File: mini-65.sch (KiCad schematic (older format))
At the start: 170 parts, among them J1 TYPE-C-31-M12_13_EDITED, J2 AVR-ISP-6, SW1 SW_Push, U1 ATmega32U4-AU, U2 USBLC6-2SC6, Y1 Crystal_GND24_Small

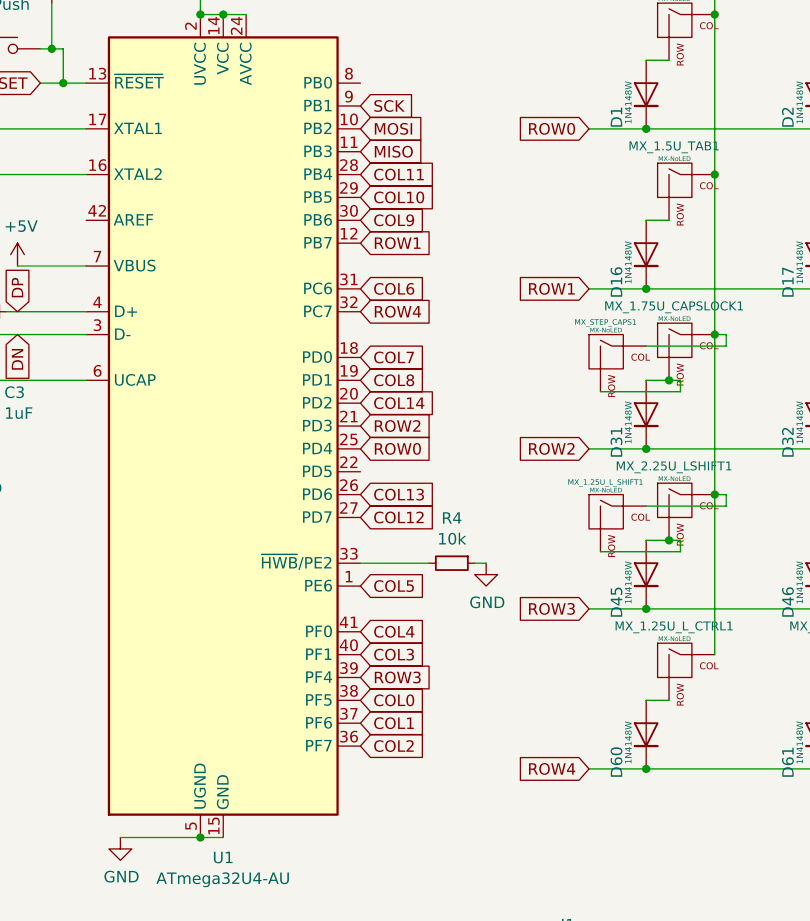
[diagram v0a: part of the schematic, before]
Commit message: misc changes, including ICSP silkscreen
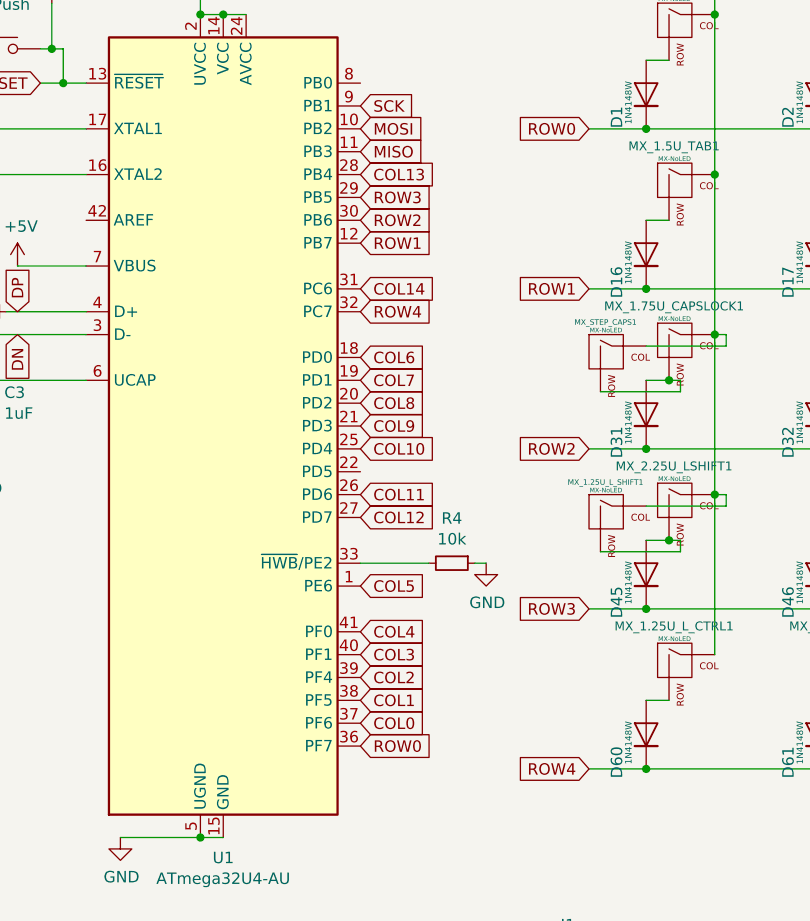
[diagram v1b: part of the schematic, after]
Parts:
- J2: footprint mini-general-tweaks:PinHeader_2x03_P2.54mm_Vertical_ICSP -> mini-general-tweaks:ICSP_2.54mm_LAYOUT
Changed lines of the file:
@@
 F 0 "J2" H 921 6596 50  0000 R CNN
 F 1 "AVR-ISP-6" H 921 6505 50  0000 R CNN
-F 2 "mini-general-tweaks:PinHeader_2x03_P2.54mm_Vertical_ICSP" V 950 6550 50  0001 C CNN
+F 2 "mini-general-tweaks:ICSP_2.54mm_LAYOUT" V 950 6550 50  0001 C CNN
 F 3 " ~" H -75 5950 50  0001 C CNN
 	1    1200 6500
@@
 	1    0    0    -1
 $EndComp
-Connection ~ 2450 1050
 Wire Wire Line
 	4200 2700 4550 2700
@@
 Wire Wire Line
 	8550 6350 8550 6400
-Text GLabel 3150 2950 2    50   Input ~ 0
-ROW0
-Text GLabel 3150 2050 2    50   Input ~ 0
-ROW1
-Text GLabel 3150 2850 2    50   Input ~ 0
-ROW2
-Text GLabel 3150 2750 2    50   Input ~ 0
-COL14
-Text GLabel 3150 3150 2    50   Input ~ 0
-COL13
-Text GLabel 3150 3250 2    50   Input ~ 0
-COL12
-Text GLabel 3150 1750 2    50   Input ~ 0
-COL11
-Text GLabel 3150 1850 2    50   Input ~ 0
-COL10
-Text GLabel 3150 1950 2    50   Input ~ 0
-COL9
-Text GLabel 3150 2650 2    50   Input ~ 0
-COL8
-Text GLabel 3150 2550 2    50   Input ~ 0
-COL7
-Text GLabel 3150 2250 2    50   Input ~ 0
-COL6
-Text GLabel 3150 2350 2    50   Input ~ 0
-ROW4
 Connection ~ 5450 3150
 Connection ~ 6500 3650
-Connection ~ 2550 1050
-Wire Wire Line
-	2650 1050 2550 1050
-Wire Wire Line
-	2550 1050 2450 1050
 Connection ~ 8300 4350
-Text GLabel 3150 4250 2    50   Input ~ 0
-COL2
-Text GLabel 3150 4150 2    50   Input ~ 0
-COL1
-Text GLabel 3150 4050 2    50   Input ~ 0
-COL0
-Text GLabel 3150 3950 2    50   Input ~ 0
-ROW3
-Text GLabel 3150 3850 2    50   Input ~ 0
-COL3
-Text GLabel 3150 3750 2    50   Input ~ 0
-COL4
-Text GLabel 3150 3550 2    50   Input ~ 0
-COL5
 Wire Wire Line
 	5450 3150 5450 3850
@@
 	5900 3650 6500 3650
 Connection ~ 4400 3650
-$Comp
-L MCU_Microchip_ATmega:ATmega32U4-AU U1
-U 1 1 5F16167A
-P 2550 2850
-F 0 "U1" H 2550 961 50  0000 C CNN
-F 1 "ATmega32U4-AU" H 2550 870 50  0000 C CNN
-F 2 "mini-general-tweaks:TQFP-44_10x10mm_P0.8mm_ATmega32U4" H 2550 2850 50  0001 C CIN
-F 3 "http://ww1.microchip.com/downloads/en/DeviceDoc/Atmel-7766-8-bit-AVR-ATmega16U4-32U4_Datasheet.pdf" H 2550 2850 50  0001 C CNN
-	1    2550 2850
-	1    0    0    -1
-$EndComp
 Wire Wire Line
 	3150 3450 3450 3450
-Connection ~ 2450 4650
-Wire Wire Line
-	2550 4650 2450 4650
-Wire Wire Line
-	2450 4650 2100 4650
 Connection ~ 5150 3650
 Wire Wire Line
@@
 	1    0    0    -1
 $EndComp
+Text GLabel 3150 3550 2    50   Input ~ 0
+COL5
+Text GLabel 3150 3750 2    50   Input ~ 0
+COL4
+Text GLabel 3150 3850 2    50   Input ~ 0
+COL3
+Text GLabel 3150 1850 2    50   Input ~ 0
+ROW3
+Text GLabel 3150 4050 2    50   Input ~ 0
+COL1
+Text GLabel 3150 4150 2    50   Input ~ 0
+COL0
+Text GLabel 3150 3950 2    50   Input ~ 0
+COL2
+Wire Wire Line
+	2450 4650 2100 4650
+Wire Wire Line
+	2550 4650 2450 4650
+Connection ~ 2450 4650
+Wire Wire Line
+	2550 1050 2450 1050
+Wire Wire Line
+	2650 1050 2550 1050
+Connection ~ 2550 1050
+Connection ~ 2450 1050
+Text GLabel 3150 4250 2    50   Input ~ 0
+ROW0
+Text GLabel 3150 2050 2    50   Input ~ 0
+ROW1
+Text GLabel 3150 1950 2    50   Input ~ 0
+ROW2
+Text GLabel 3150 2250 2    50   Input ~ 0
+COL14
+Text GLabel 3150 3250 2    50   Input ~ 0
+COL12
+Text GLabel 3150 3150 2    50   Input ~ 0
+COL11
+Text GLabel 3150 2950 2    50   Input ~ 0
+COL10
+Text GLabel 3150 2850 2    50   Input ~ 0
+COL9
+Text GLabel 3150 2750 2    50   Input ~ 0
+COL8
+Text GLabel 3150 2650 2    50   Input ~ 0
+COL7
+Text GLabel 3150 2550 2    50   Input ~ 0
+COL6
+Text GLabel 3150 2350 2    50   Input ~ 0
+ROW4
+$Comp
+L MCU_Microchip_ATmega:ATmega32U4-AU U1
+U 1 1 5F16167A
+P 2550 2850
+F 0 "U1" H 2550 961 50  0000 C CNN
+F 1 "ATmega32U4-AU" H 2550 870 50  0000 C CNN
+F 2 "mini-general-tweaks:TQFP-44_10x10mm_P0.8mm_ATmega32U4" H 2550 2850 50  0001 C CIN
+F 3 "http://ww1.microchip.com/downloads/en/DeviceDoc/Atmel-7766-8-bit-AVR-ATmega16U4-32U4_Datasheet.pdf" H 2550 2850 50  0001 C CNN
+	1    2550 2850
+	1    0    0    -1
+$EndComp
+Text GLabel 3150 1750 2    50   Input ~ 0
+COL13
 $EndSCHEMATC
